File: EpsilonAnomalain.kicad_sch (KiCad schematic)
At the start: 79 parts, among them J1 I2C, J2 ServoA, J3 ServoB, J4 ServoC, J5 ServoD, J6 USB_C, SW1 ON, U1 ESP32-S3FN8, U10 USBLC6-2SC6, U2 ICM-42688-P, U3 BMP388, U4 AHT20, U5 W25N01GVZEIG, U6 KCSA02-105, U7 74HC595, U8 TPS61088, U9 AP2112K-3.3, Y1 40 MHz

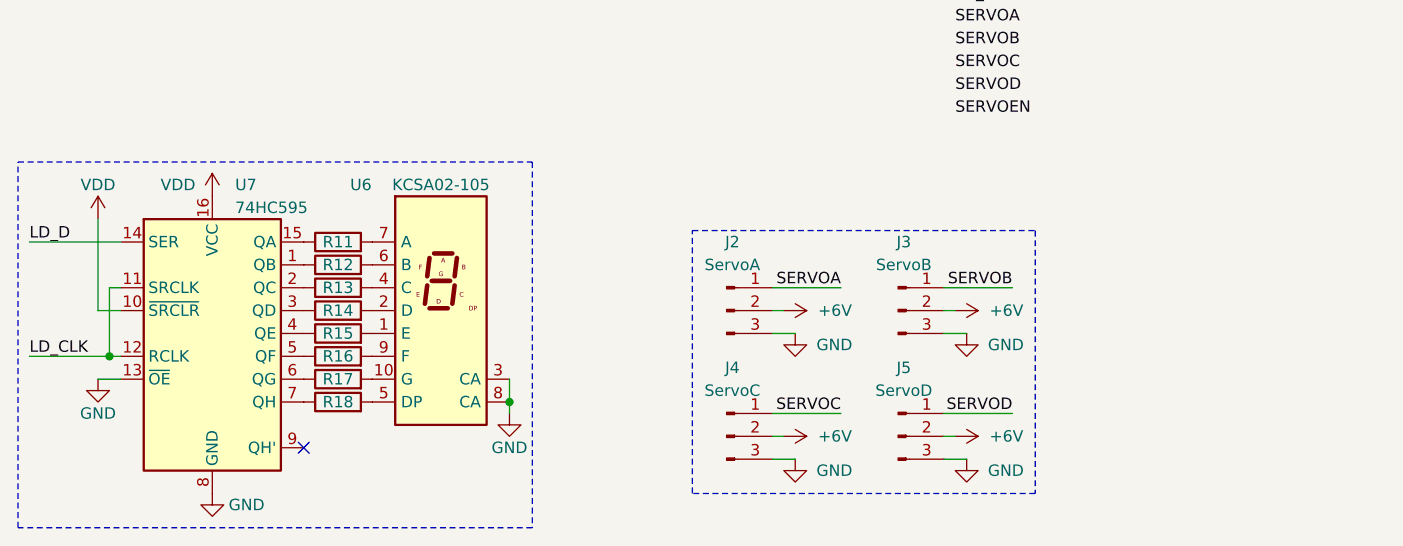
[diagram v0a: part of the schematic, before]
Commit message: rev2.10
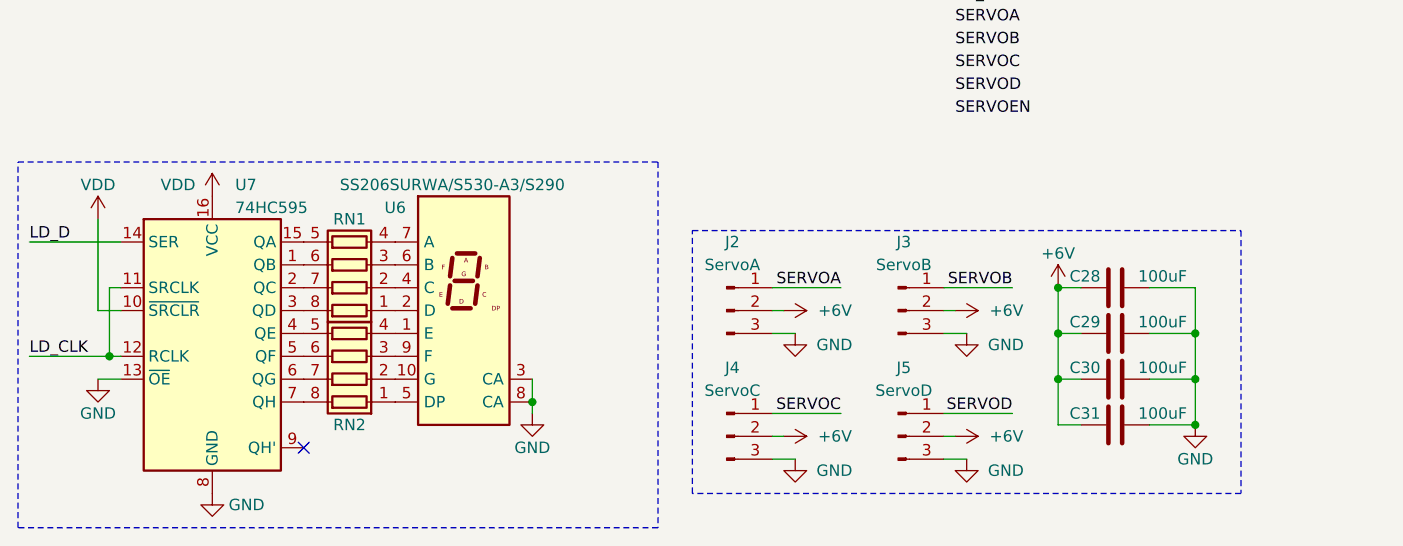
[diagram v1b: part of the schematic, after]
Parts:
- removed R11, R12, R13, R14, R15, R16, R17, R18: 1k, Resistor_SMD:R_0402_1005Metric, symbol Device:R
- added C28, C29, C30, C31: 100uF, Capacitor_SMD:C_1206_3216Metric, symbol Device:C
- added RN1, RN2: 1k, Resistor_SMD:R_Array_Convex_4x0402, symbol Device:R_Pack04
- C26, C27: footprint (none) -> Capacitor_SMD:C_1206_3216Metric
- U6: value KCSA02-105 -> SS206SURWA/S530-A3/S290; footprint Display_7Segment:KCSC02-105 -> CustomPackage:SS206SURWA
- U7: footprint Package_SO:SO-16_3.9x9.9mm_P1.27mm -> Package_SO:TSSOP-16_4.4x5mm_P0.65mm
- U8: footprint (none) -> UltraLibrarian:RHL0020A
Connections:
- net +6V: now also C28.1, C29.1, C30.1, C31.1
- net GND: now also C28.2, C29.2, C30.2, C31.2
- net at U7.3 (QD): now also RN1.8 (R1.2)
- net at U6.2 (D): now also RN1.1 (R1.1)
- net at U7.6 (QG): now also RN2.7 (R2.2)
- net at U6.10 (G): now also RN2.2 (R2.1)
- net at U7.7 (QH): now also RN2.8 (R1.2)
- net at U6.5 (DP): now also RN2.1 (R1.1)
- net at U7.15 (QA): now also RN1.5 (R4.2)
- net at U6.7 (A): now also RN1.4 (R4.1)
- net at U6.1 (E): now also RN2.4 (R4.1)
- net at U6.4 (C): now also RN1.2 (R2.1)
- net at U6.6 (B): now also RN1.3 (R3.1)
- net at U6.9 (F): now also RN2.3 (R3.1)
- net at U7.2 (QC): now also RN1.7 (R2.2)
- net at U7.1 (QB): now also RN1.6 (R3.2)
- net at U7.4 (QE): now also RN2.5 (R4.2)
- net at U7.5 (QF): now also RN2.6 (R3.2)
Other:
- moved on the sheet: U6

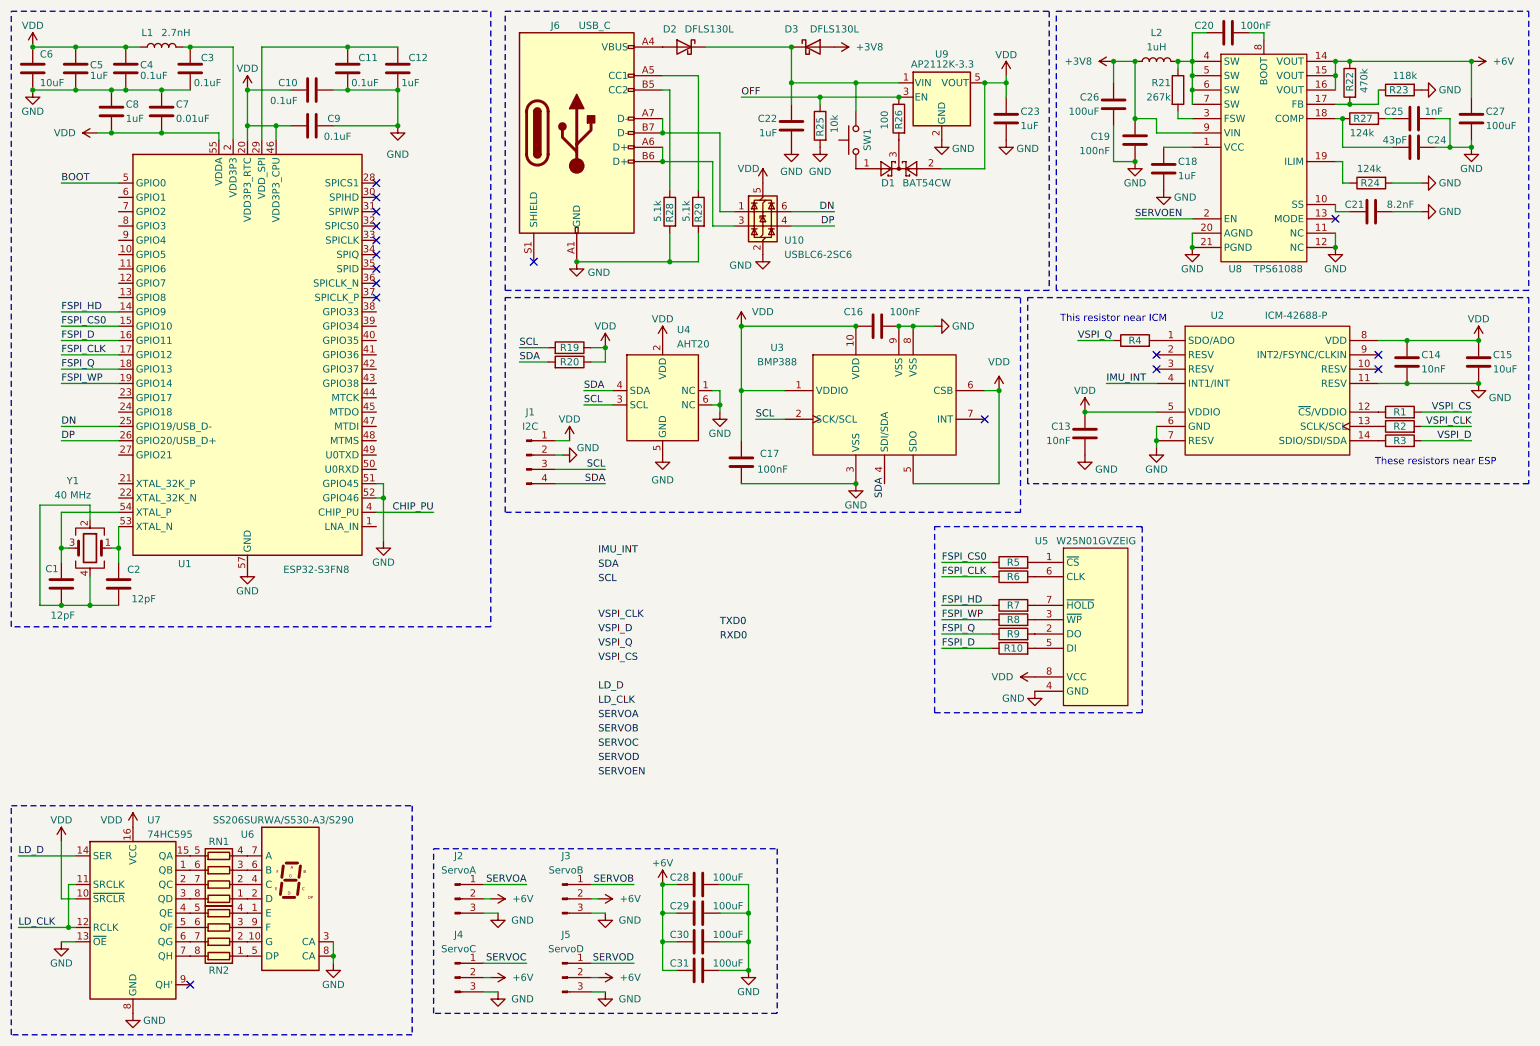
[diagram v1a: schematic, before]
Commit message: v2.13
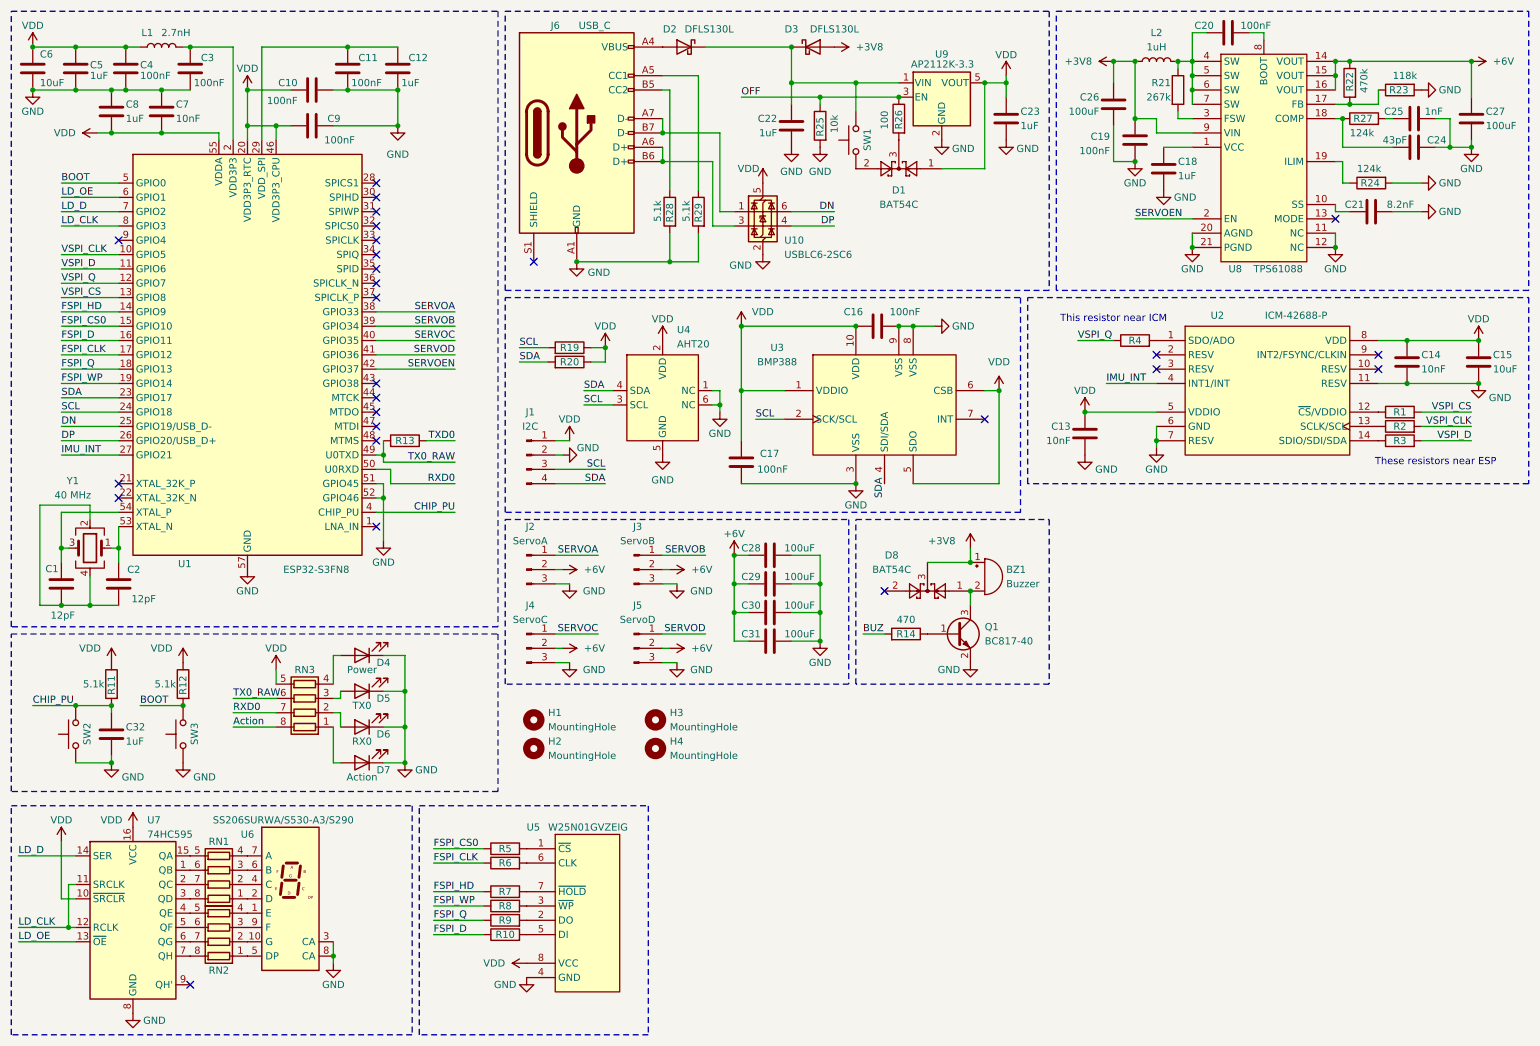
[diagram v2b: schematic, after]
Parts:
- removed D1: BAT54CW, Package_TO_SOT_SMD:SOT-323_SC-70, symbol Diode:BAT54CW
- added BZ1: Buzzer, Buzzer_Beeper:MagneticBuzzer_CUI_CMT-8504-100-SMT, symbol Device:Buzzer
- added C32: 1uF, Capacitor_SMD:C_0402_1005Metric, symbol Device:C
- added D1, D8: BAT54C, Package_TO_SOT_SMD:SOT-23, symbol Diode:BAT54C
- added D4: Power, LED_SMD:LED_0402_1005Metric, symbol Device:LED
- added D5: TX0, LED_SMD:LED_0402_1005Metric, symbol Device:LED
- added D6: RX0, LED_SMD:LED_0402_1005Metric, symbol Device:LED
- added D7: Action, LED_SMD:LED_0402_1005Metric, symbol Device:LED
- added H1, H2, H3, H4: MountingHole, MountingHole:MountingHole_3.2mm_M3_Pad_Via, symbol Mechanical:MountingHole
- added Q1: BC817-40, Package_TO_SOT_SMD:SOT-23, symbol Transistor_BJT:BC817
- added R11, R12: 5.1k, Resistor_SMD:R_0402_1005Metric, symbol Device:R
- added R13, R14: 470, Resistor_SMD:R_0402_1005Metric, symbol Device:R
- added RN3: 1k, Resistor_SMD:R_Array_Convex_4x0402, symbol Device:R_Pack04
- added SW2, SW3: ON, Button_Switch_SMD:SW_SPST_TL3342, symbol Switch:SW_Push
- C10, C11, C3, C4, C9: value 0.1uF -> 100nF
- C7: value 0.01uF -> 10nF
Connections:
- net +3V8: now also BZ1.1 (+), D8.3
- net BOOT: now also R12.2, SW3.2
- net CHIP_PU: now also C32.1, R11.2, SW2.2
- net GND: now also C32.2, D4.1 (K), D5.1 (K), D6.1 (K), D7.1 (K), Q1.2 (E), SW2.1, SW3.1; no longer U7.13 (~{OE})
- net IMU_INT: now also U1.27 (GPIO21)
- net LD_CLK: now also U1.8 (GPIO3)
- net LD_D: now also U1.7 (GPIO2)
- net RXD0: now also U1.50 (U0RXD), RN3.7 (R2.2)
- net SCL: now also U1.24 (GPIO18)
- net SDA: now also U1.23 (GPIO17)
- net SERVOA: now also U1.38 (GPIO33)
- net SERVOB: now also U1.39 (GPIO34)
- net SERVOC: now also U1.40 (GPIO35)
- net SERVOD: now also U1.41 (GPIO36)
- net SERVOEN: now also U1.42 (GPIO37)
- net TXD0: now also R13.1
- net VDD: now also D1.1, R11.1, R12.1, RN3.5 (R4.2)
- net VSPI_CLK: now also U1.10 (GPIO5)
- net VSPI_CS: now also U1.13 (GPIO8)
- net VSPI_D: now also U1.11 (GPIO6)
- net VSPI_Q: now also U1.12 (GPIO7)
- net TX0_RAW: now reaches U1.49 (U0TXD)
- net TX0_RAW: now also R13.2, RN3.6 (R3.2)
- net LD_OE: now reaches U1.6 (GPIO1)
- net LD_OE: now also U7.13 (~{OE})
- net at R26.2: now also D1.3
- net at SW1.1: now also D1.2
- new net: Q1.1 (B), R14.1
- new net: D4.2 (A), RN3.4 (R4.1)
- new net: D6.2 (A), RN3.2 (R2.1)
- new net: BZ1.2 (-), D8.1, Q1.3 (C)
- new net: D7.2 (A), RN3.1 (R1.1)
- new net: D5.2 (A), RN3.3 (R3.1)
- new net Action: RN3.8 (R1.2)
- new net BUZ: R14.2
- no-connect marks 17 -> 27
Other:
- moved on the sheet: C28, C29, C30, C31, J2, J3, J4, J5, R10, R5, R6, R7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

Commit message: v2.14
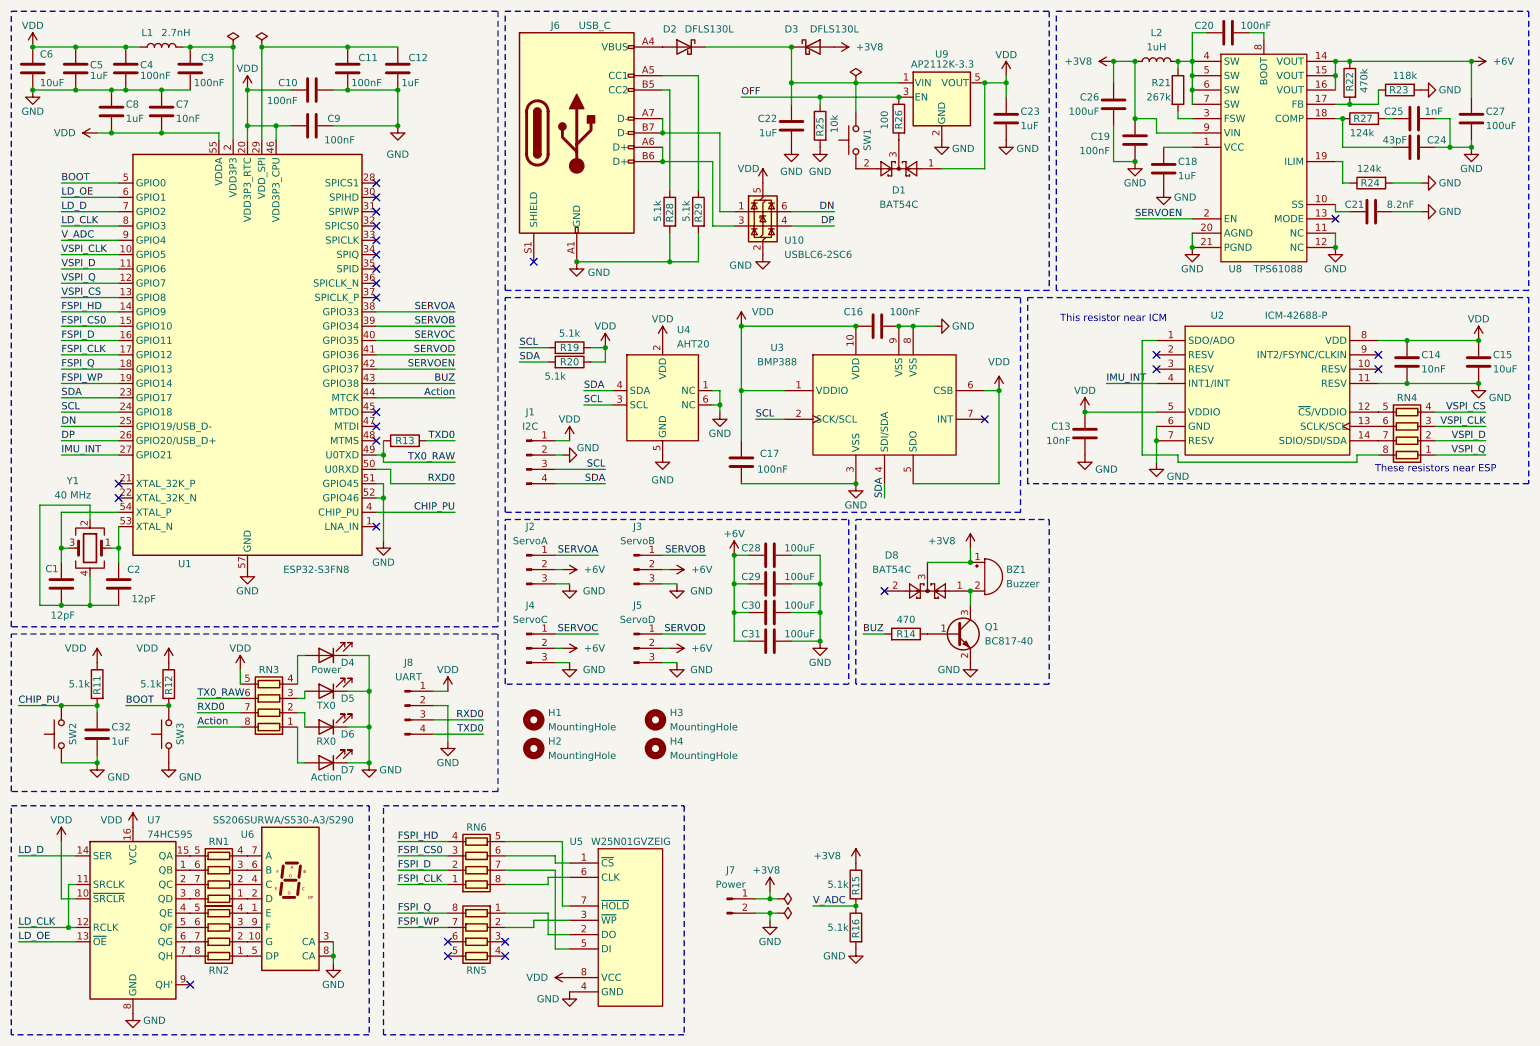
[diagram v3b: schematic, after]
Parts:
- removed R1, R2, R3, R4: 100, Resistor_SMD:R_0402_1005Metric, symbol Device:R
- removed R10, R5, R6, R7, R8, R9: 0, Resistor_SMD:R_0402_1005Metric, symbol Device:R
- added J7: Power, CustomConnectors:Battery_3V7_Cable_connector_v2, symbol Connector:Conn_01x02_Pin
- added J8: UART, Connector_JST:JST_XH_B4B-XH-A_1x04_P2.50mm_Vertical, symbol Connector:Conn_01x04_Pin
- added R15, R16: 5.1k, Resistor_SMD:R_0402_1005Metric, symbol Device:R
- added RN4: 100, Resistor_SMD:R_Array_Convex_4x0402, symbol Device:R_Pack04
- added RN5, RN6: 0, Resistor_SMD:R_Array_Convex_4x0402, symbol Device:R_Pack04
- L2: footprint Capacitor_SMD:C_0402_1005Metric -> Inductor_SMD:L_APV_APH0630
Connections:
- net +3V8: now also J7.1 (Pin_1), R15.1
- net Action: now also U1.44 (MTCK)
- net BUZ: now also U1.43 (GPIO38)
- net FSPI_CLK: now also RN6.1 (R1.1)
- net FSPI_CS0: now also RN6.3 (R3.1)
- net FSPI_D: now also RN6.2 (R2.1)
- net FSPI_HD: now also RN6.4 (R4.1)
- net FSPI_Q: now also RN5.8 (R1.2)
- net FSPI_WP: now also RN5.7 (R2.2)
- net GND: now also J7.2 (Pin_2), J8.2 (Pin_2), R16.2
- net RXD0: now also J8.3 (Pin_3)
- net SDA: now also U3.4 (SDI/SDA)
- net TXD0: now also J8.4 (Pin_4)
- net VDD: now also J8.1 (Pin_1)
- net VSPI_CLK: now also RN4.3 (R3.1)
- net VSPI_CS: now also RN4.4 (R4.1)
- net VSPI_D: now also RN4.2 (R2.1)
- net VSPI_Q: now also RN4.1 (R1.1)
- net at U2.13 (SCLK/SCL): now also RN4.6 (R3.2)
- net at U2.1 (SDO/ADO): now also RN4.8 (R1.2)
- net at U2.12 (~{CS}/VDDIO): now also RN4.5 (R4.2)
- net at U2.14 (SDIO/SDI/SDA): now also RN4.7 (R2.2)
- net V_ADC: now reaches U1.9 (GPIO4)
- net V_ADC: now also R15.2, R16.1
- net at U5.1 (~{CS}): now also RN6.6 (R3.2)
- net at U5.2 (DO): now also RN5.1 (R1.1)
- net at U5.3 (~{WP}): now also RN5.2 (R2.1)
- net at U5.5 (DI): now also RN6.7 (R2.2)
- net at U5.6 (CLK): now also RN6.8 (R1.2)
- net at U5.7 (~{HOLD}): now also RN6.5 (R4.2)
- no-connect marks 27 -> 28
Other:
- moved on the sheet: C32, D4, D5, D6, D7, R11, R12, RN3, SW2, SW3, U5
